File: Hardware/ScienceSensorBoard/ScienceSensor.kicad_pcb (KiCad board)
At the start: 2 copper layers, 2 x 2 mm, 93 parts, among them J1 Conn_02x03_Counter_Clockwise, J2 RJ45_LED_Shielded, Q1 SI4156DY, Q10 BSS138, Q11 SI4156DY, Q2 SI4156DY, Q3 SI4156DY, Q4 BSS138, Q5 BSS138, Q6 BSS138, Q7 BSS138, Q8 BSS138, Q9 BSS138, U1 TSR_1-2450, U2 OKI-78SR-3.3_1.5-W36H-C, U3 Teensy4.1_DEV-16771, U6 IRS2005S, U7 IRS2005S

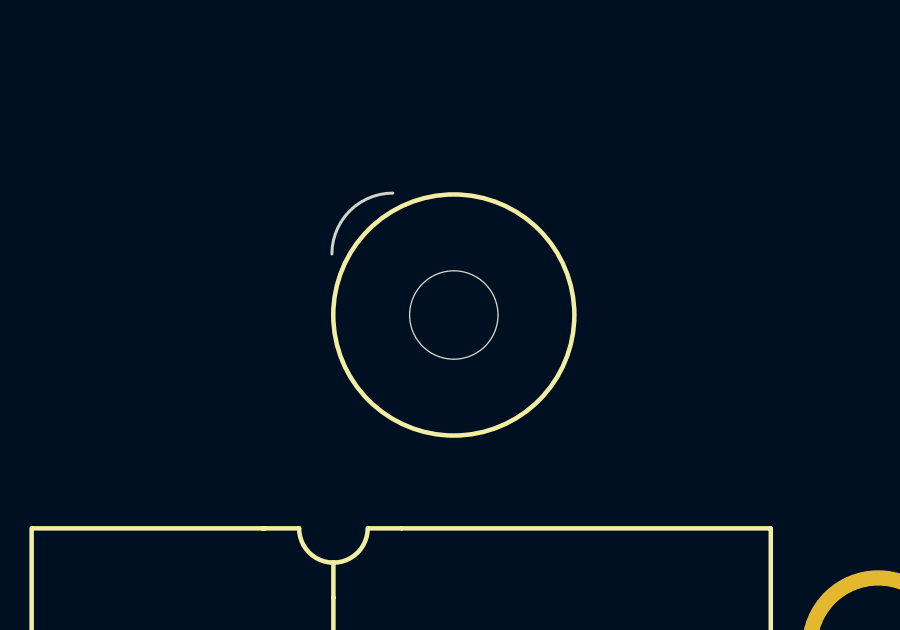
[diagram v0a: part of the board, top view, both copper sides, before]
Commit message: Layout Organization
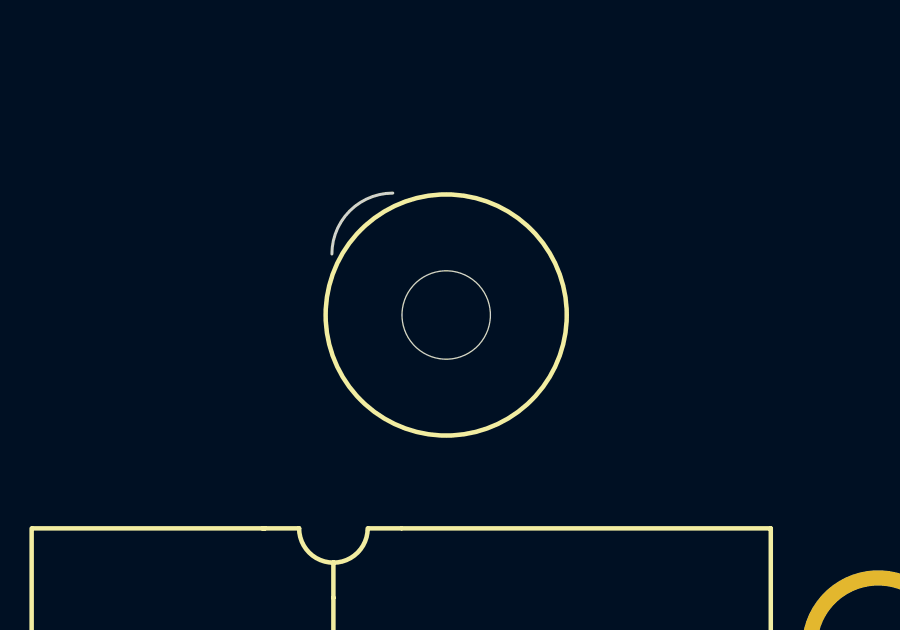
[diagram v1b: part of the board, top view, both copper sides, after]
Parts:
- moved V1 0.25 mm to (147.3, 66.3)
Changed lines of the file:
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@@
   )
   (footprint "MRDT_Drill_Holes:4_40_Hole" (layer "F.Cu")
-    (at 147.574 66.294)
+    (at 147.32 66.294)
     (property "Sheetfile" "ScienceSensor.kicad_sch")
     (property "Sheetname" "")
